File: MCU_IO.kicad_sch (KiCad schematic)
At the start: 27 parts, among them J1 Conn_02x07_Odd_Even, J10 Conn_01x05, U7 TMS320F28379DPTPQ, U8 M24512, U9 MAX809, Y1 10 MHz

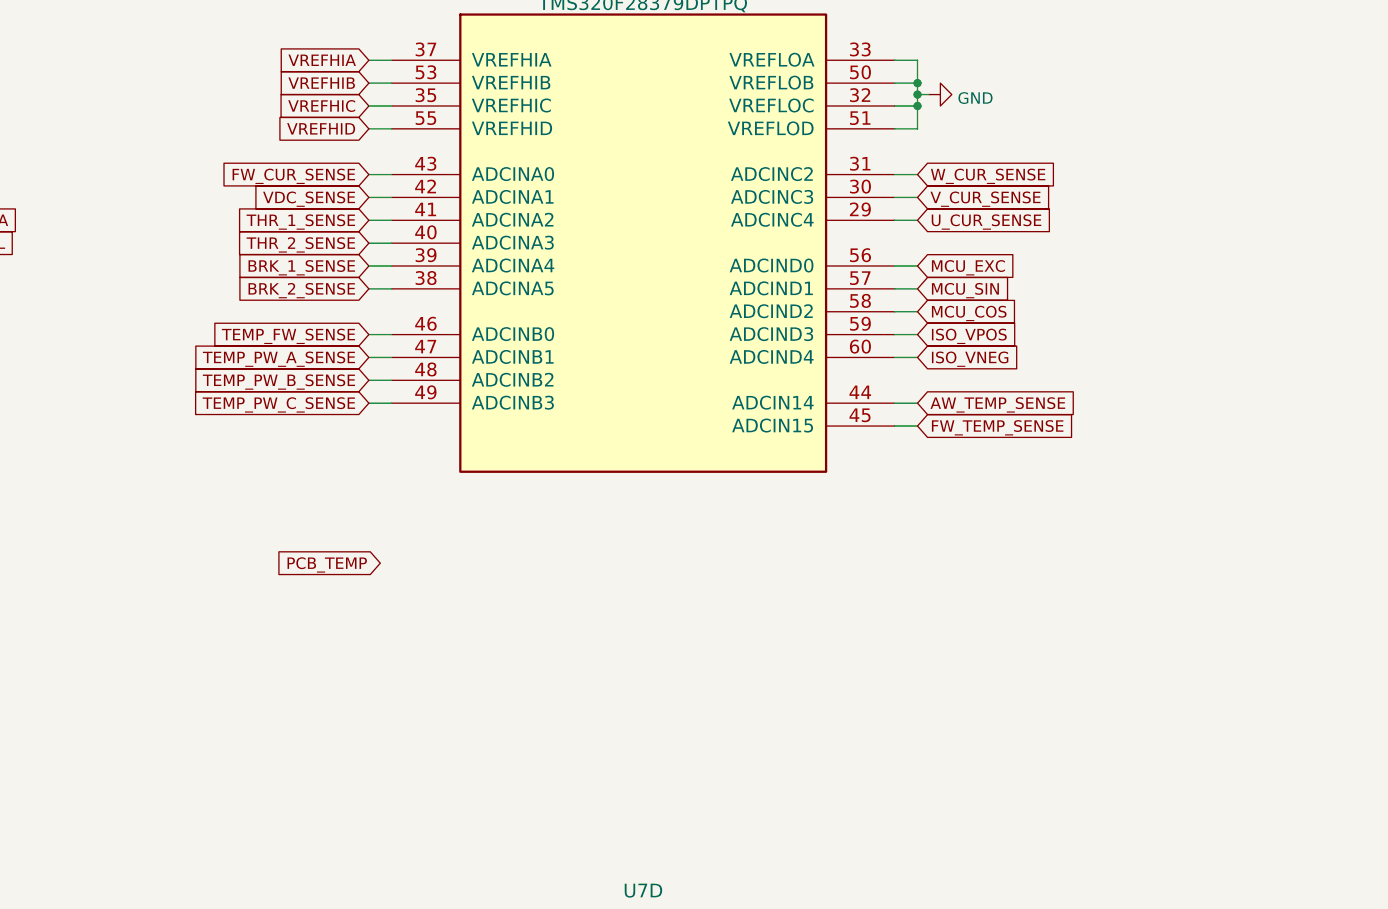
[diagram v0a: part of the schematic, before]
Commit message: Добавления: Расставил все на плате
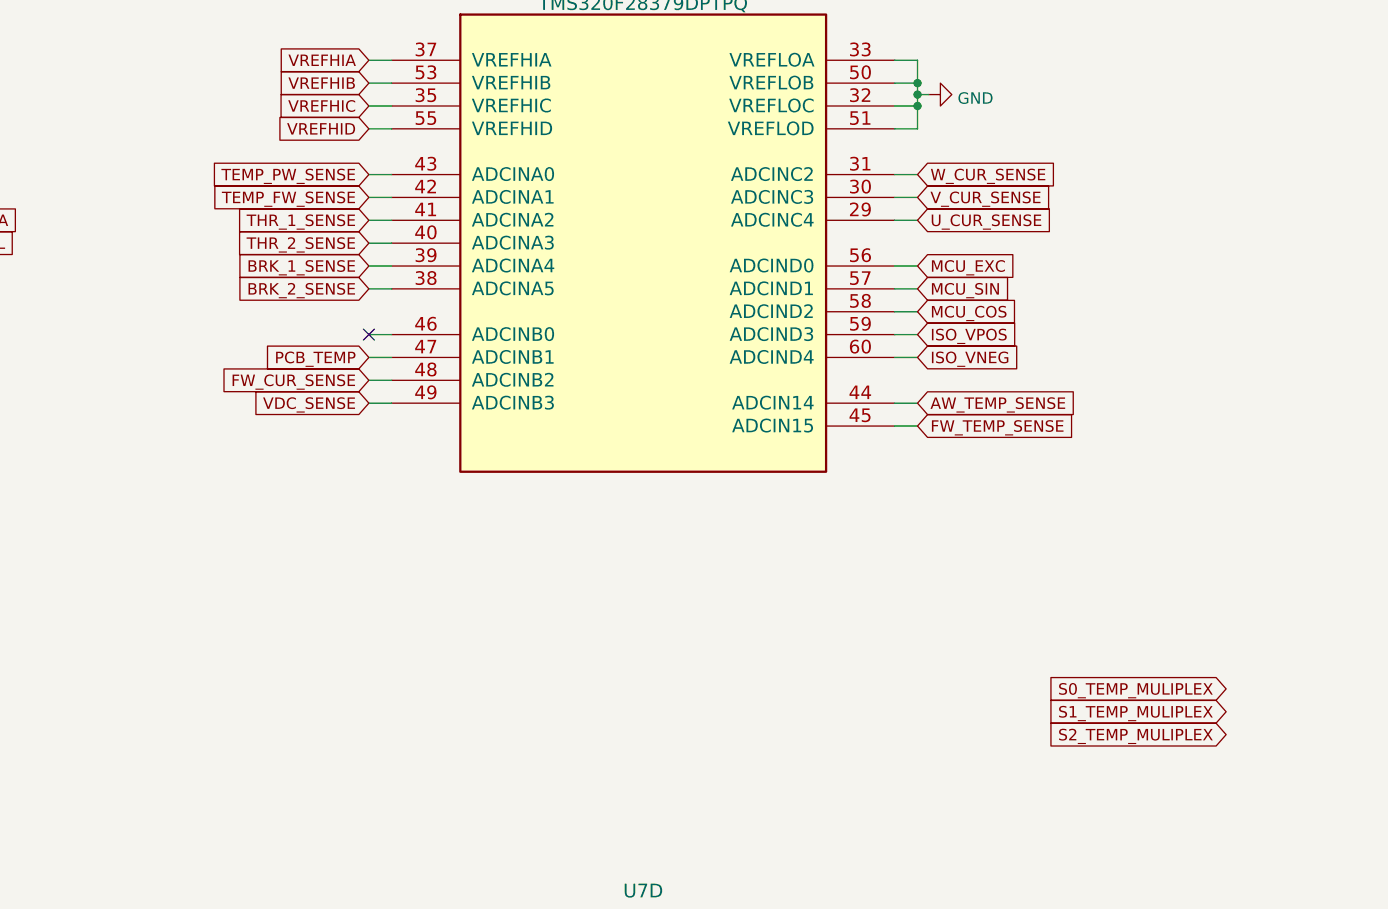
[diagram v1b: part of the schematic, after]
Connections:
- net TEMP_PW_A_SENSE is gone; now on net PCB_TEMP: U7.47 (ADCINB1)
- net TEMP_PW_B_SENSE is gone; now on net FW_CUR_SENSE: U7.48 (ADCINB2)
- net TEMP_PW_C_SENSE is gone; now on net VDC_SENSE: U7.49 (ADCINB3)
- net FW_CUR_SENSE: no longer U7.43 (ADCINA0)
- net TEMP_FW_SENSE: now also U7.42 (ADCINA1); no longer U7.46 (ADCINB0)
- net VDC_SENSE: no longer U7.42 (ADCINA1)
- new net TEMP_PW_SENSE: U7.43 (ADCINA0)
- no-connect marks 10 -> 11
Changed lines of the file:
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@@
 	)
 	(no_connect
+		(at 179.07 73.66)
+	)
+	(no_connect
 		(at 198.12 224.79)
 	)
@@
 		)
 	)
-	(global_label "TEMP_PW_B_SENSE"
+	(global_label "GPIO42"
 		(shape input)
-		(at 179.07 78.74 180)
+		(at 125.73 86.36 0)
 		(fields_autoplaced yes)
 		(effects
@@
 				(size 1.27 1.27)
 			)
-			(justify right)
+			(justify left)
 		)
 		(property "Intersheetrefs" "${INTERSHEET_REFS}"
-			(at 158.3051 78.74 0)
+			(at 135.0374 86.2806 0)
 			(effects
 				(font
 					(size 1.27 1.27)
 				)
-				(justify right)
+				(justify left)
 				(hide yes)
 			)
 		)
 	)
-	(global_label "GPIO42"
+	(global_label "S0_TEMP_MULIPLEX"
 		(shape input)
-		(at 125.73 86.36 0)
+		(at 274.32 113.03 180)
 		(fields_autoplaced yes)
 		(effects
@@
 				(size 1.27 1.27)
 			)
-			(justify left)
+			(justify right)
 		)
 		(property "Intersheetrefs" "${INTERSHEET_REFS}"
-			(at 135.0374 86.2806 0)
+			(at 253.0712 113.03 0)
 			(effects
 				(font
 					(size 1.27 1.27)
 				)
-				(justify left)
+				(justify right)
 				(hide yes)
 			)
@@
 	(global_label "TEMP_FW_SENSE"
 		(shape input)
-		(at 179.07 73.66 180)
+		(at 179.07 58.42 180)
 		(fields_autoplaced yes)
 		(effects
@@
 		)
 		(property "Intersheetrefs" "${INTERSHEET_REFS}"
-			(at 161.2959 73.7394 0)
+			(at 161.2959 58.4994 0)
 			(effects
 				(font
@@
 	(global_label "VDC_SENSE"
 		(shape input)
-		(at 179.07 58.42 180)
+		(at 179.07 81.28 180)
 		(fields_autoplaced yes)
 		(effects
@@
 		)
 		(property "Intersheetrefs" "${INTERSHEET_REFS}"
-			(at 166.0131 58.4994 0)
+			(at 166.0131 81.3594 0)
 			(effects
 				(font
@@
 	(global_label "FW_CUR_SENSE"
 		(shape input)
-		(at 179.07 55.88 180)
+		(at 179.07 78.74 180)
 		(fields_autoplaced yes)
 		(effects
@@
 		)
 		(property "Intersheetrefs" "${INTERSHEET_REFS}"
-			(at 162.2636 55.8006 0)
+			(at 162.2636 78.6606 0)
 			(effects
 				(font
@@
 		)
 	)
-	(global_label "OSC_OUT"
+	(global_label "S1_TEMP_MULIPLEX"
 		(shape input)
-		(at 181.61 149.86 180)
+		(at 274.32 115.57 180)
 		(fields_autoplaced yes)
 		(effects
@@
 		)
 		(property "Intersheetrefs" "${INTERSHEET_REFS}"
-			(at 170.7907 149.7806 0)
+			(at 253.0712 115.57 0)
 			(effects
 				(font
@@
 		)
 	)
-	(global_label "TEMP_PW_C_SENSE"
+	(global_label "OSC_OUT"
 		(shape input)
-		(at 179.07 81.28 180)
+		(at 181.61 149.86 180)
 		(fields_autoplaced yes)
 		(effects
@@
 		)
 		(property "Intersheetrefs" "${INTERSHEET_REFS}"
-			(at 158.3051 81.28 0)
+			(at 170.7907 149.7806 0)
 			(effects
 				(font
@@
 		)
 	)
-	(global_label "TEMP_PW_A_SENSE"
+	(global_label "TEMP_PW_SENSE"
 		(shape input)
-		(at 179.07 76.2 180)
+		(at 179.07 55.88 180)
 		(fields_autoplaced yes)
 		(effects
@@
 		)
 		(property "Intersheetrefs" "${INTERSHEET_REFS}"
-			(at 158.4865 76.2 0)
+			(at 160.5427 55.88 0)
 			(effects
 				(font
@@
 	(global_label "PCB_TEMP"
 		(shape input)
-		(at 180.34 99.06 180)
+		(at 179.07 76.2 180)
 		(fields_autoplaced yes)
 		(effects
@@
 		)
 		(property "Intersheetrefs" "${INTERSHEET_REFS}"
-			(at 167.7392 99.06 0)
+			(at 166.4692 76.2 0)
 			(effects
 				(font
@@
 				(hide yes)
 			)
+		)
+	)
+	(global_label "S2_TEMP_MULIPLEX"
+		(shape input)
+		(at 274.32 118.11 180)
+		(fields_autoplaced yes)
+		(effects
+			(font
+				(size 1.27 1.27)
+			)
+			(justify right)
+		)
+		(property "Intersheetrefs" "${INTERSHEET_REFS}"
+			(at 253.0712 118.11 0)
+			(effects
+				(font
+					(size 1.27 1.27)
+				)
+				(justify right)
+				(hide yes)
+			)
